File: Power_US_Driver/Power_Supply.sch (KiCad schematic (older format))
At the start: 6 parts, among them T1 Transformer_1P_1S, U1 LM7805_TO220

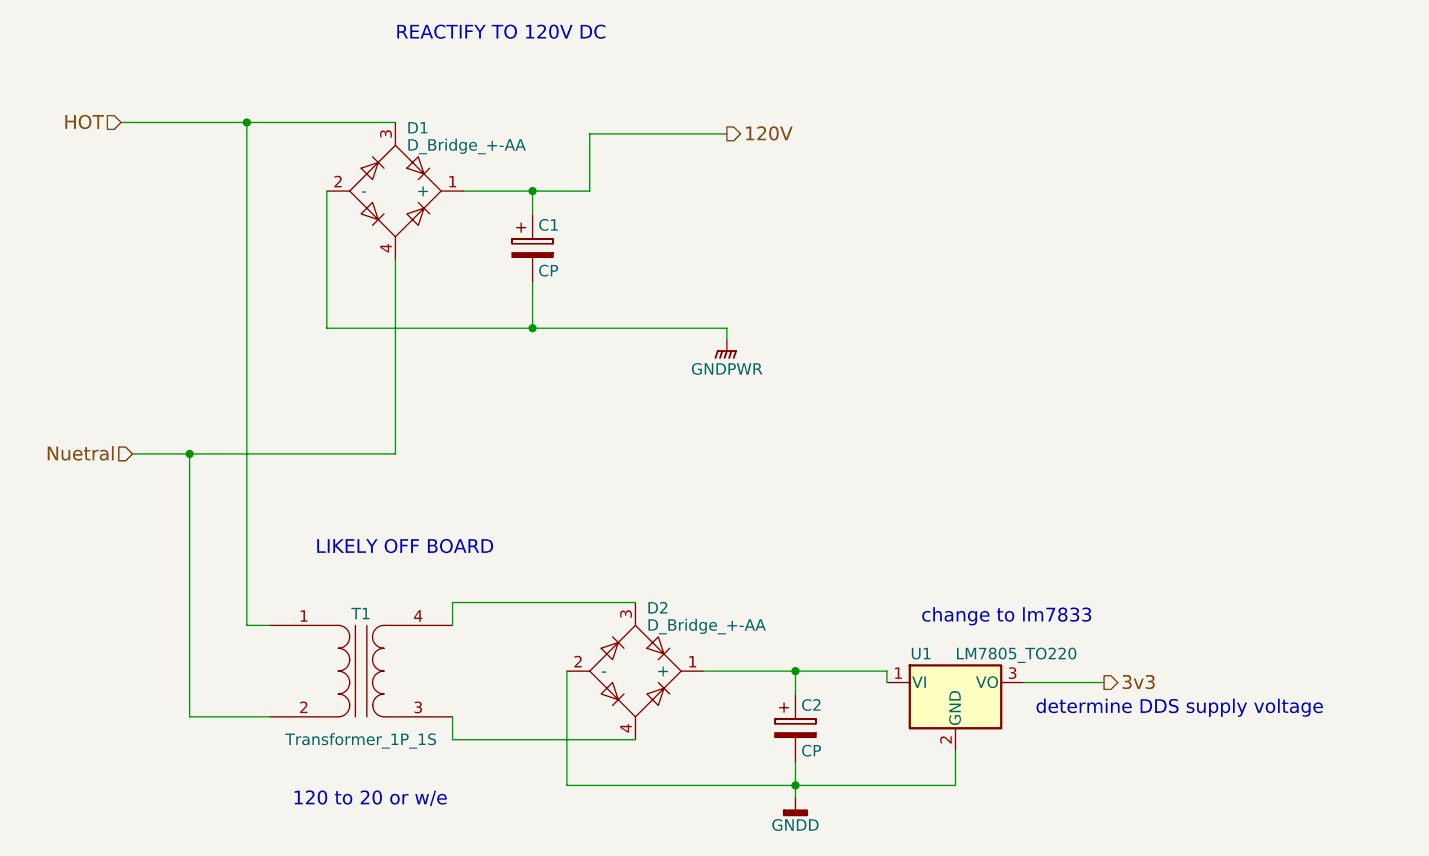
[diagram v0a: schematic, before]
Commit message: initial Current sense more vacilating over power drive solution
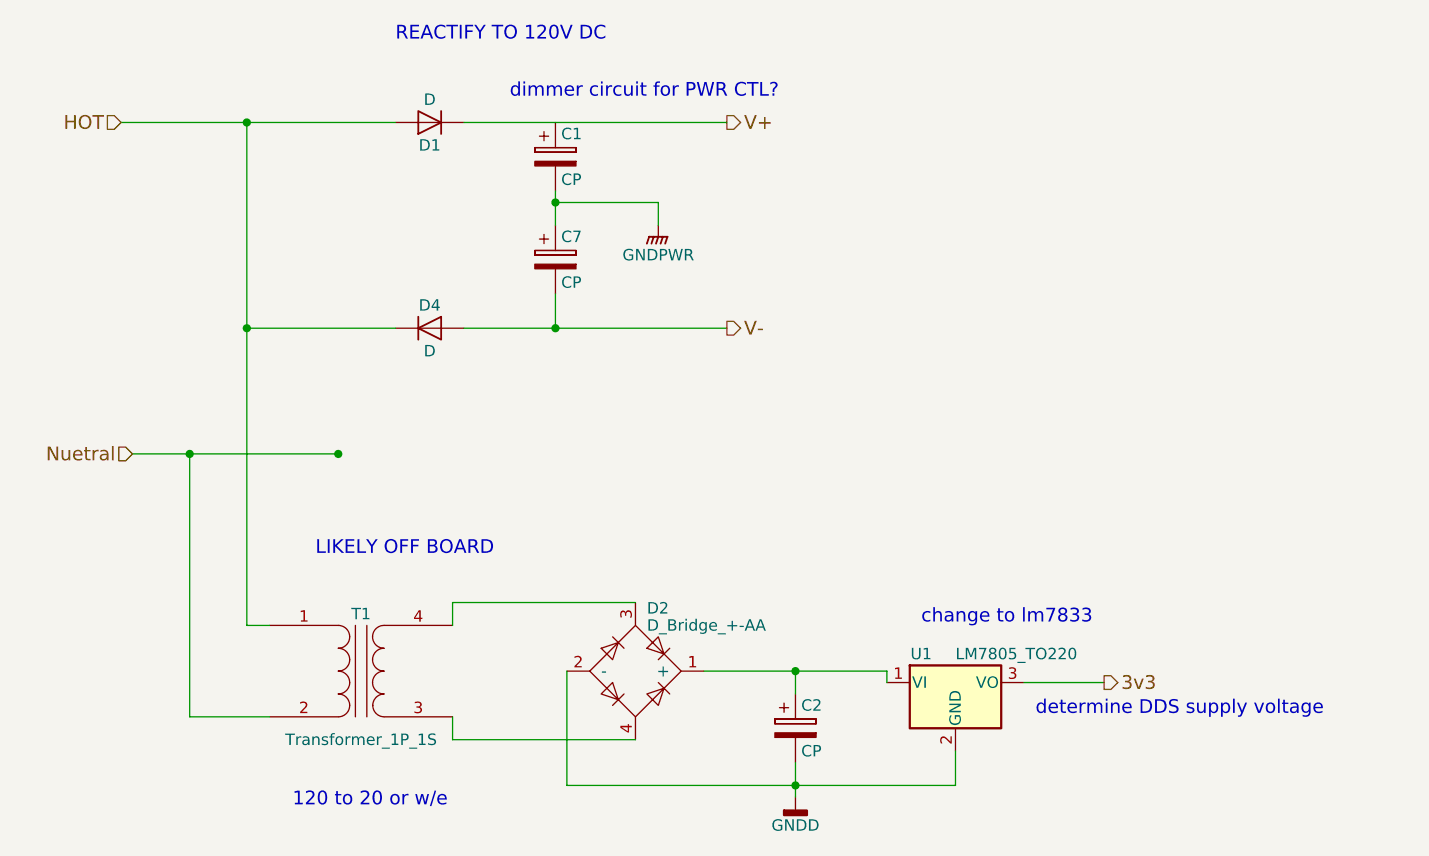
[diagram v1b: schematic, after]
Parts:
- removed D1: D_Bridge_+-AA, symbol D_Bridge_+-AA
- added C7: CP, symbol CP
- added D1, D4: D, symbol D
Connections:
- net GNDPWR: now also C7.1
- net HOT: now also D1.2 (A), D4.1 (K)
- net 120V: no longer names the net of C1.1
- new net V+: D1.1 (K)
- new net V-: C7.2, D4.2 (A)
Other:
- note added: "dimmer circuit for PWR CTL?"
- moved on the sheet: C1
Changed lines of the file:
@@
 120 to 20 or w/e
-$Comp
-L D_Bridge_+-AA D1
-U 1 1 5AAD8E46
-P 2250 2300
-F 0 "D1" H 2300 2575 50  0000 L CNN
-F 1 "D_Bridge_+-AA" H 2300 2500 50  0000 L CNN
-F 2 "" H 2250 2300 50  0001 C CNN
-F 3 "" H 2250 2300 50  0001 C CNN
-	1    2250 2300
-	1    0    0    -1
-$EndComp
 $Comp
 L D_Bridge_+-AA D2
@@
 	1    0    0    -1
 $EndComp
-Text HLabel 3700 2050 2    60   Output ~ 0
-120V
+Text HLabel 3700 2000 2    60   Output ~ 0
+V+
 Text HLabel 1050 2000 0    60   Input ~ 0
 HOT
@@
 Wire Wire Line
 	1050 2000 2250 2000
-Wire Wire Line
-	2250 3450 2250 2600
-Wire Wire Line
-	1100 3450 2250 3450
-Wire Wire Line
-	2550 2300 3100 2300
-Wire Wire Line
-	3100 2300 3100 2050
-Wire Wire Line
-	3100 2050 3700 2050
-Wire Wire Line
-	1950 2300 1950 2900
-Wire Wire Line
-	1950 2900 3700 2900
 Wire Wire Line
 	1700 4200 1600 4200
@@
 L CP C1
 U 1 1 5AAE86CA
-P 2850 2550
-F 0 "C1" H 2875 2650 50  0000 L CNN
-F 1 "CP" H 2875 2450 50  0000 L CNN
-F 2 "" H 2888 2400 50  0001 C CNN
-F 3 "" H 2850 2550 50  0001 C CNN
-	1    2850 2550
+P 2950 2150
+F 0 "C1" H 2975 2250 50  0000 L CNN
+F 1 "CP" H 2975 2050 50  0000 L CNN
+F 2 "" H 2988 2000 50  0001 C CNN
+F 3 "" H 2950 2150 50  0001 C CNN
+	1    2950 2150
 	1    0    0    -1
 $EndComp
-Wire Wire Line
-	2850 2400 2850 2300
-Connection ~ 2850 2300
-Wire Wire Line
-	2850 2700 2850 2900
-Connection ~ 2850 2900
 $Comp
 L CP C2
@@
 Connection ~ 4000 4900
 $Comp
-L GNDPWR #PWR2
+L GNDPWR #PWR4
 U 1 1 5AB00CEA
-P 3700 2950
-F 0 "#PWR2" H 3700 2750 50  0001 C CNN
-F 1 "GNDPWR" H 3700 2820 50  0000 C CNN
-F 2 "" H 3700 2900 50  0001 C CNN
-F 3 "" H 3700 2900 50  0001 C CNN
-	1    3700 2950
+P 3400 2450
+F 0 "#PWR4" H 3400 2250 50  0001 C CNN
+F 1 "GNDPWR" H 3400 2320 50  0000 C CNN
+F 2 "" H 3400 2400 50  0001 C CNN
+F 3 "" H 3400 2400 50  0001 C CNN
+	1    3400 2450
 	1    0    0    -1
 $EndComp
-Wire Wire Line
-	3700 2900 3700 2950
 $Comp
-L GNDD #PWR3
+L GNDD #PWR5
 U 1 1 5AB013C1
 P 4000 4950
-F 0 "#PWR3" H 4000 4700 50  0001 C CNN
+F 0 "#PWR5" H 4000 4700 50  0001 C CNN
 F 1 "GNDD" H 4000 4825 50  0000 C CNN
 F 2 "" H 4000 4950 50  0001 C CNN
@@
 Text Notes 4550 4200 0    60   ~ 0
 change to lm7833
+$Comp
+L D D1
+U 1 1 5AB252E8
+P 2400 2000
+F 0 "D1" H 2400 2100 50  0000 C CNN
+F 1 "D" H 2400 1900 50  0000 C CNN
+F 2 "" H 2400 2000 50  0001 C CNN
+F 3 "" H 2400 2000 50  0001 C CNN
+	1    2400 2000
+	-1   0    0    1
+$EndComp
+$Comp
+L D D4
+U 1 1 5AB2532E
+P 2400 2900
+F 0 "D4" H 2400 3000 50  0000 C CNN
+F 1 "D" H 2400 2800 50  0000 C CNN
+F 2 "" H 2400 2900 50  0001 C CNN
+F 3 "" H 2400 2900 50  0001 C CNN
+	1    2400 2900
+	1    0    0    -1
+$EndComp
+Text HLabel 3700 2900 2    60   Output ~ 0
+V-
+Wire Wire Line
+	3700 2000 2550 2000
+$Comp
+L CP C7
+U 1 1 5AB2577F
+P 2950 2600
+F 0 "C7" H 2975 2700 50  0000 L CNN
+F 1 "CP" H 2975 2500 50  0000 L CNN
+F 2 "" H 2988 2450 50  0001 C CNN
+F 3 "" H 2950 2600 50  0001 C CNN
+	1    2950 2600
+	1    0    0    -1
+$EndComp
+Wire Wire Line
+	2950 2300 2950 2450
+Wire Wire Line
+	2950 2750 2950 2900
+Wire Wire Line
+	2550 2900 3700 2900
+Wire Wire Line
+	3400 2450 3400 2350
+Wire Wire Line
+	3400 2350 2950 2350
+Connection ~ 2950 2350
+Connection ~ 2950 2900
+Wire Wire Line
+	1600 2900 2250 2900
+Connection ~ 2000 3450
+Wire Wire Line
+	2000 3450 1100 3450
+Connection ~ 1600 2900
+Text Notes 2750 1900 0    60   ~ 0
+dimmer circuit for PWR CTL?
 $EndSCHEMATC
